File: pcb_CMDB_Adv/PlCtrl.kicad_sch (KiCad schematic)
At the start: 34 parts, among them IC2 Wio-SX1262, SW3 SW_RESET, SW4 SW_BOOT, U5 ESP32-WROOM-32UE, U7 MCP23017_SO

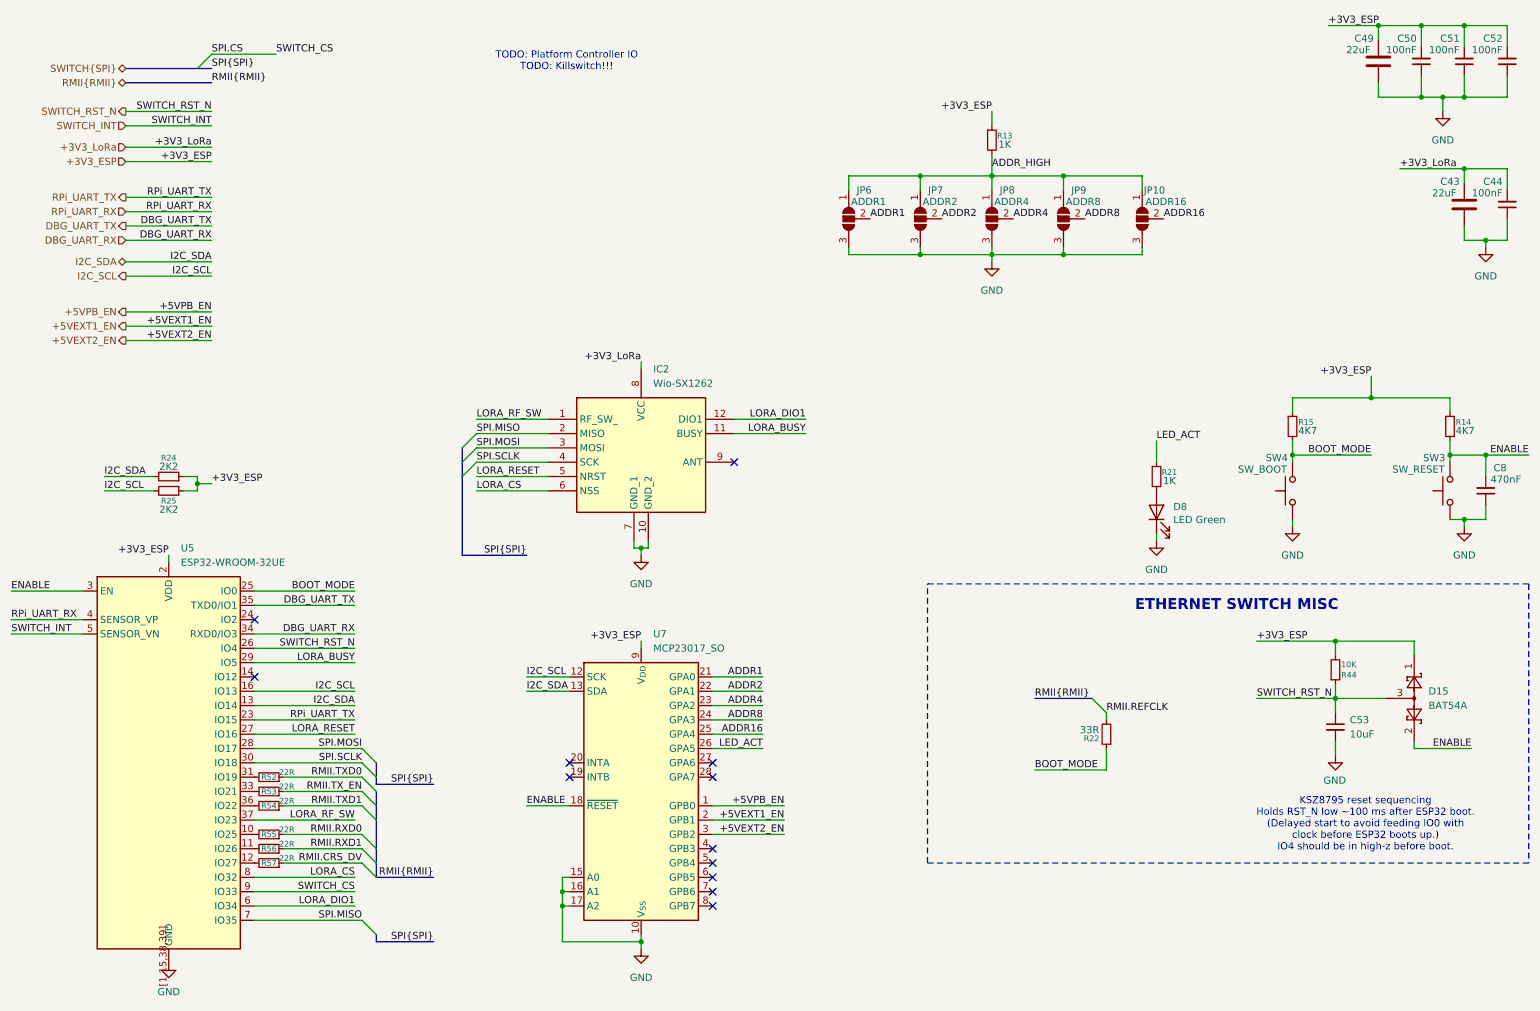
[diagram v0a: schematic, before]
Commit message: WIP
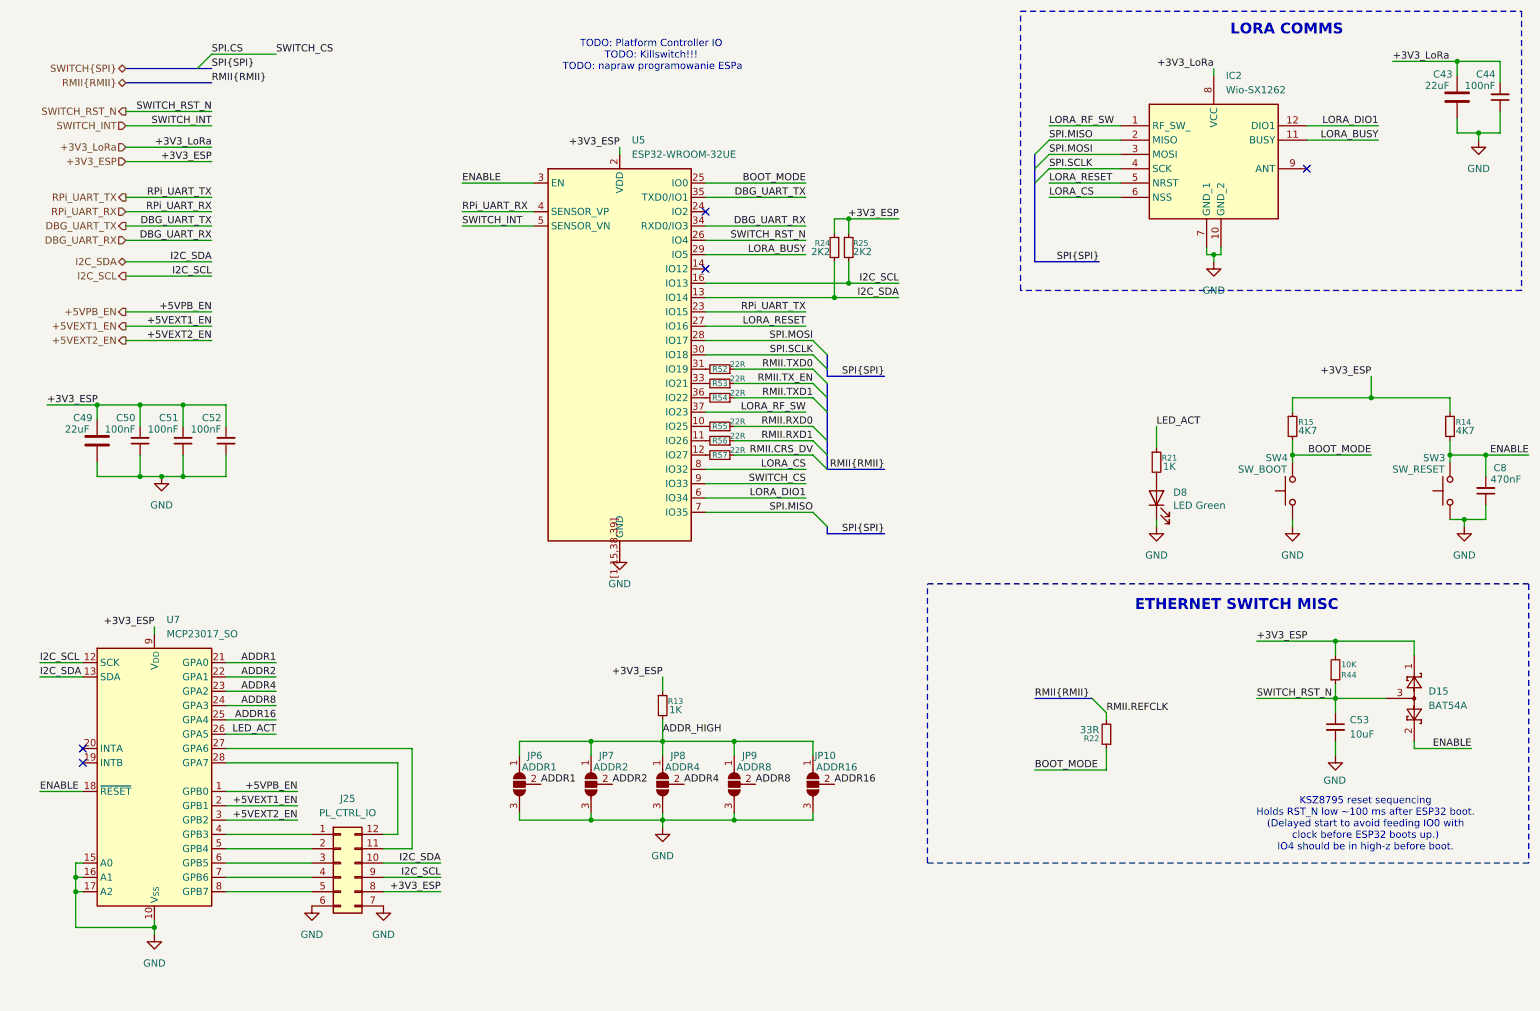
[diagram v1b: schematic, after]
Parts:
- added J25: PL_CTRL_IO, symbol Connector_Generic:Conn_02x06_Counter_Clockwise
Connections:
- net +3V3_ESP: now also J25.8 (Pin_8)
- net GND: now also J25.6 (Pin_6), J25.7 (Pin_7)
- net I2C_SCL: now also J25.9 (Pin_9)
- net I2C_SDA: now also J25.10 (Pin_10)
- net at U7.27 (GPA6): now also J25.11 (Pin_11)
- net at U7.28 (GPA7): now also J25.12 (Pin_12)
- net at U7.4 (GPB3): now also J25.1 (Pin_1)
- net at U7.5 (GPB4): now also J25.2 (Pin_2)
- net at U7.6 (GPB5): now also J25.3 (Pin_3)
- net at U7.7 (GPB6): now also J25.4 (Pin_4)
- net at U7.8 (GPB7): now also J25.5 (Pin_5)
- no-connect marks 12 -> 5
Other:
- note added: "LORA COMMS"
- note added: "TODO: napraw programowanie ESPa"
- moved on the sheet: C43, C44, C49, C50, C51, C52, D8, IC2, JP10, JP6, JP7, JP8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
